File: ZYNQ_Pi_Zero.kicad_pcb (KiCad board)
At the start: 4 copper layers, 35 parts, among them Q501 2N7002, Q502 2N7002, Q503 2N7002, U101 xc7z010clg400, U201 MT41K256M16TW-107_P, U301 W25Q256FVEI, U501 TPD4E05U06DQA, U502 TPD4E05U06DQA

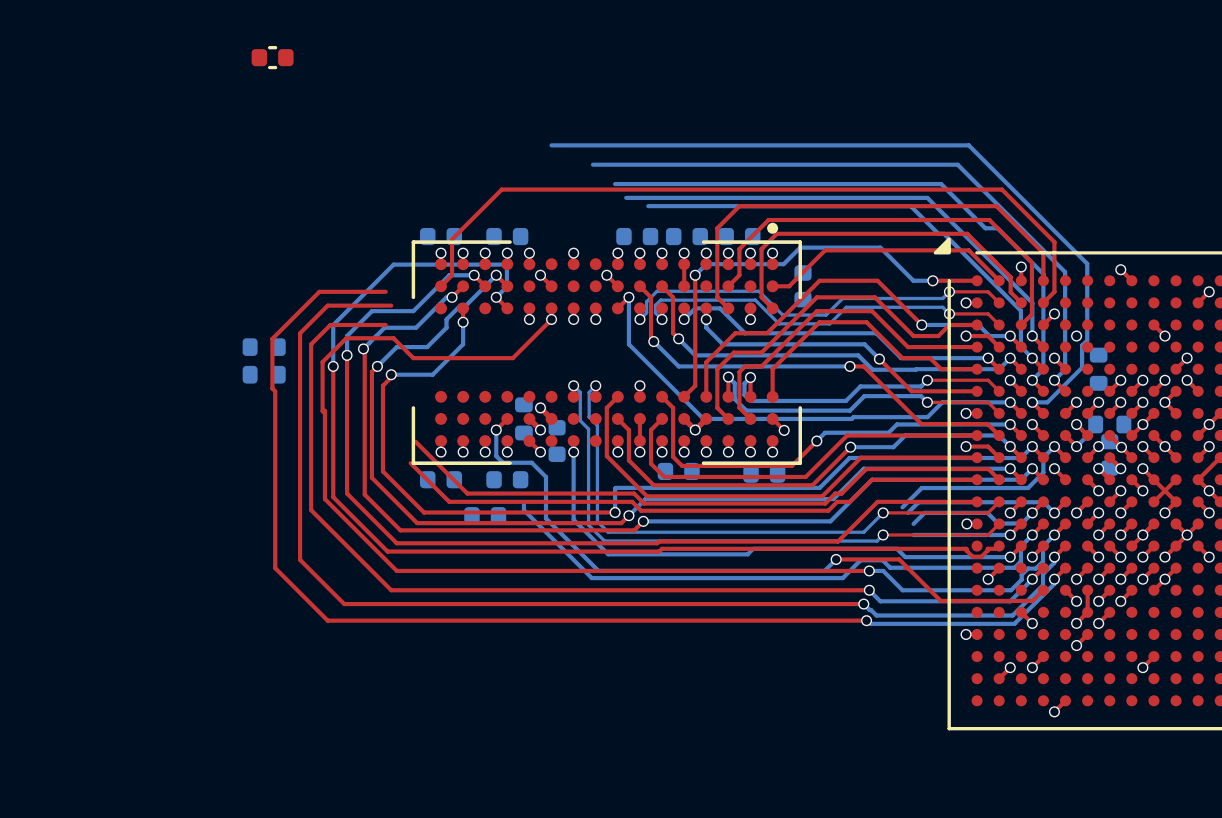
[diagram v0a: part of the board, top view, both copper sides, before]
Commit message: feat: continue routing ddr
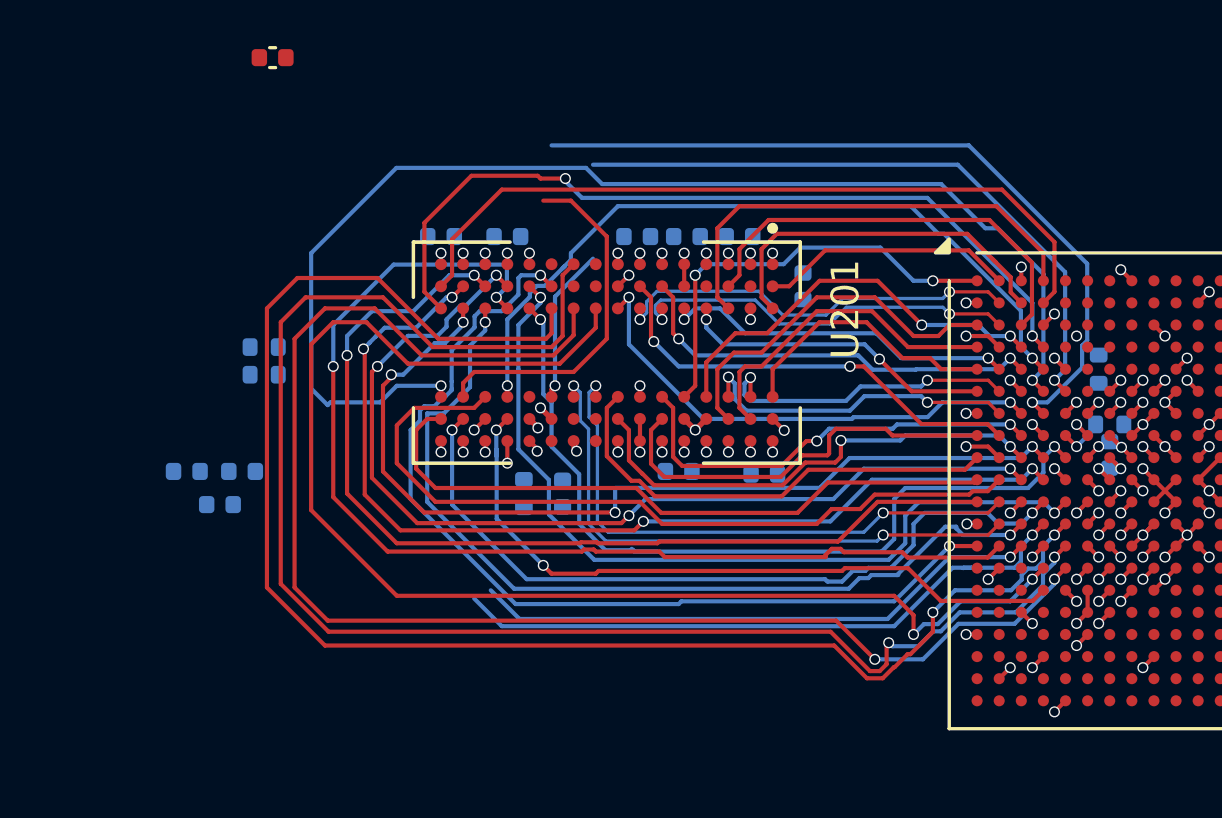
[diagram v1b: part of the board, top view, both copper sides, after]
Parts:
- moved C210 9.61 mm to (114.0, 100.5)
- moved C209 9.60 mm to (114.8, 99.3)
- moved C214 9.20 mm to (112.8, 99.3)
- moved R201 2.70 mm to (125.0, 100.1)
- moved C206 1.91 mm to (126.4, 100.1)
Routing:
- net /DDR3/DDR_~{CS}: track 0.57 -> 34.7 mm, vias 1 -> 2
- net /DDR3/DDR_A2: track 4.07 -> 32.3 mm, vias 1 -> 2
- net /DDR3/DDR_BA0: track 6.19 -> 30.4 mm, vias 1 -> 2
- net /DDR3/DDR_A14: track 21.4 -> 44.5 mm, vias 1 -> 2
- net /DDR3/DDR_A6: track 5.35 -> 27.8 mm, vias 1 -> 2
- net /DDR3/DDR_BA2: track 7.70 -> 29.5 mm
- net /DDR3/DDR_ODT: track 42.2 -> 56.2 mm, vias 3 -> 2
- net /DDR3/DDR_A11: track 27.9 -> 40.8 mm
- net /DDR3/DDR_A13: track 18.0 -> 29.8 mm, vias 1 -> 2
- net /DDR3/DDR_~{WE}: track 44.6 -> 56.2 mm, vias 3 -> 2
- net /DDR3/DDR_~{RAS}: track 37.8 -> 48.3 mm, vias 3 -> 2
- net /DDR3/DDR_A12: track 17.5 -> 27.4 mm, vias 1 -> 2
- net /DDR3/DDR_~{CAS}: track 43.9 -> 52.0 mm, vias 3 -> 2
- net /DDR3/DDR_A1: track 22.7 -> 28.4 mm
- net /DDR3/DDR_A10: track 23.3 -> 29.0 mm, vias 1 -> 2
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
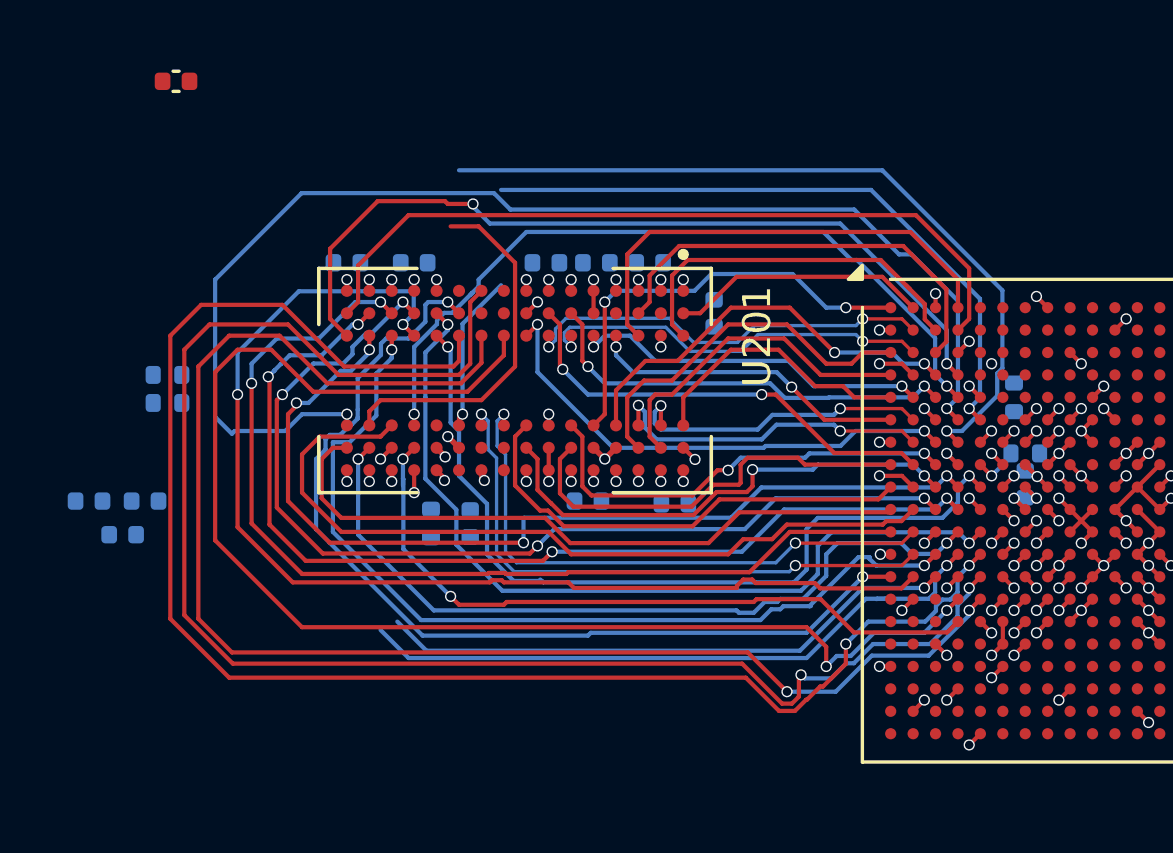
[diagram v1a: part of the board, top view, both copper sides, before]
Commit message: feat: continue routing ddr
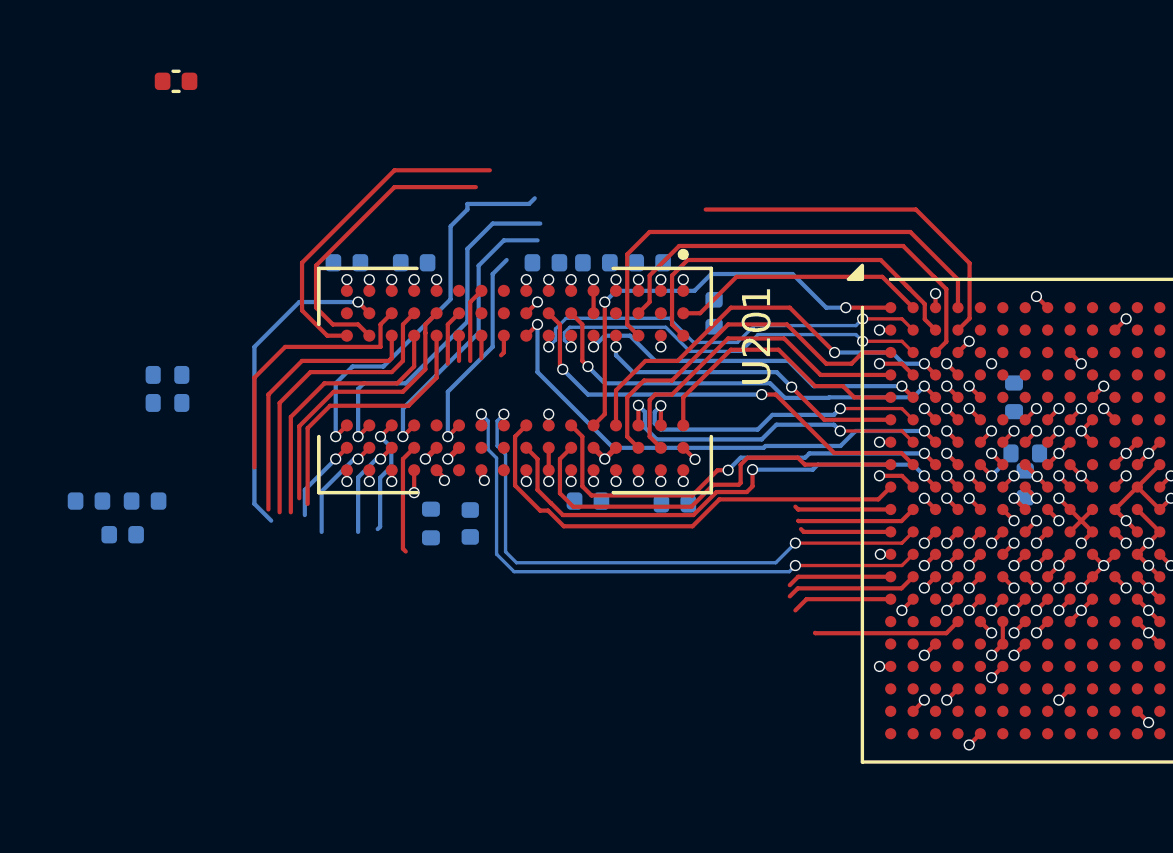
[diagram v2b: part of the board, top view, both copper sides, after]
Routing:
- net /DDR3/DDR_~{WE}: track 56.2 -> 1.47 mm, vias 2 -> 1
- net /DDR3/DDR_ODT: track 56.2 -> 3.23 mm, vias 2 -> 1
- net /DDR3/DDR_~{CAS}: track 52.0 -> 1.37 mm, vias 2 -> 1
- net /DDR3/DDR_~{RAS}: track 48.3 -> 1.31 mm, vias 2 -> 1
- net /DDR3/DDR_A14: track 44.5 -> 14.5 mm
- net /DDR3/DDR_~{CS}: track 34.7 -> 5.69 mm, vias 2 -> 0
- net /DDR3/DDR_A11: track 40.8 -> 13.3 mm, vias 1 -> 2
- net /DDR3/DDR_A0: track 40.8 -> 14.3 mm, vias 2 -> 0
- net /DDR3/DDR_A3: track 35.7 -> 11.4 mm, vias 4 -> 1
- net /DDR3/DDR_A7: track 36.0 -> 11.9 mm, vias 4 -> 2
- net /DDR3/DDR_A6: track 27.8 -> 4.35 mm
- net /DDR3/DDR_A5: track 36.0 -> 12.8 mm, vias 2 -> 0
- net /DDR3/DDR_A9: track 33.7 -> 11.2 mm, vias 4 -> 1
- net /DDR3/DDR_A2: track 32.3 -> 10.4 mm, vias 2 -> 1
- net /DDR3/DDR_A10: track 29.0 -> 8.30 mm
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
